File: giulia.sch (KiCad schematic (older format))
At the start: 128 parts, among them J1 AVR-ISP-6, SW1 RESET, SW2 BOOT, U1 ATmega32A-PU, Y1 16 MHz

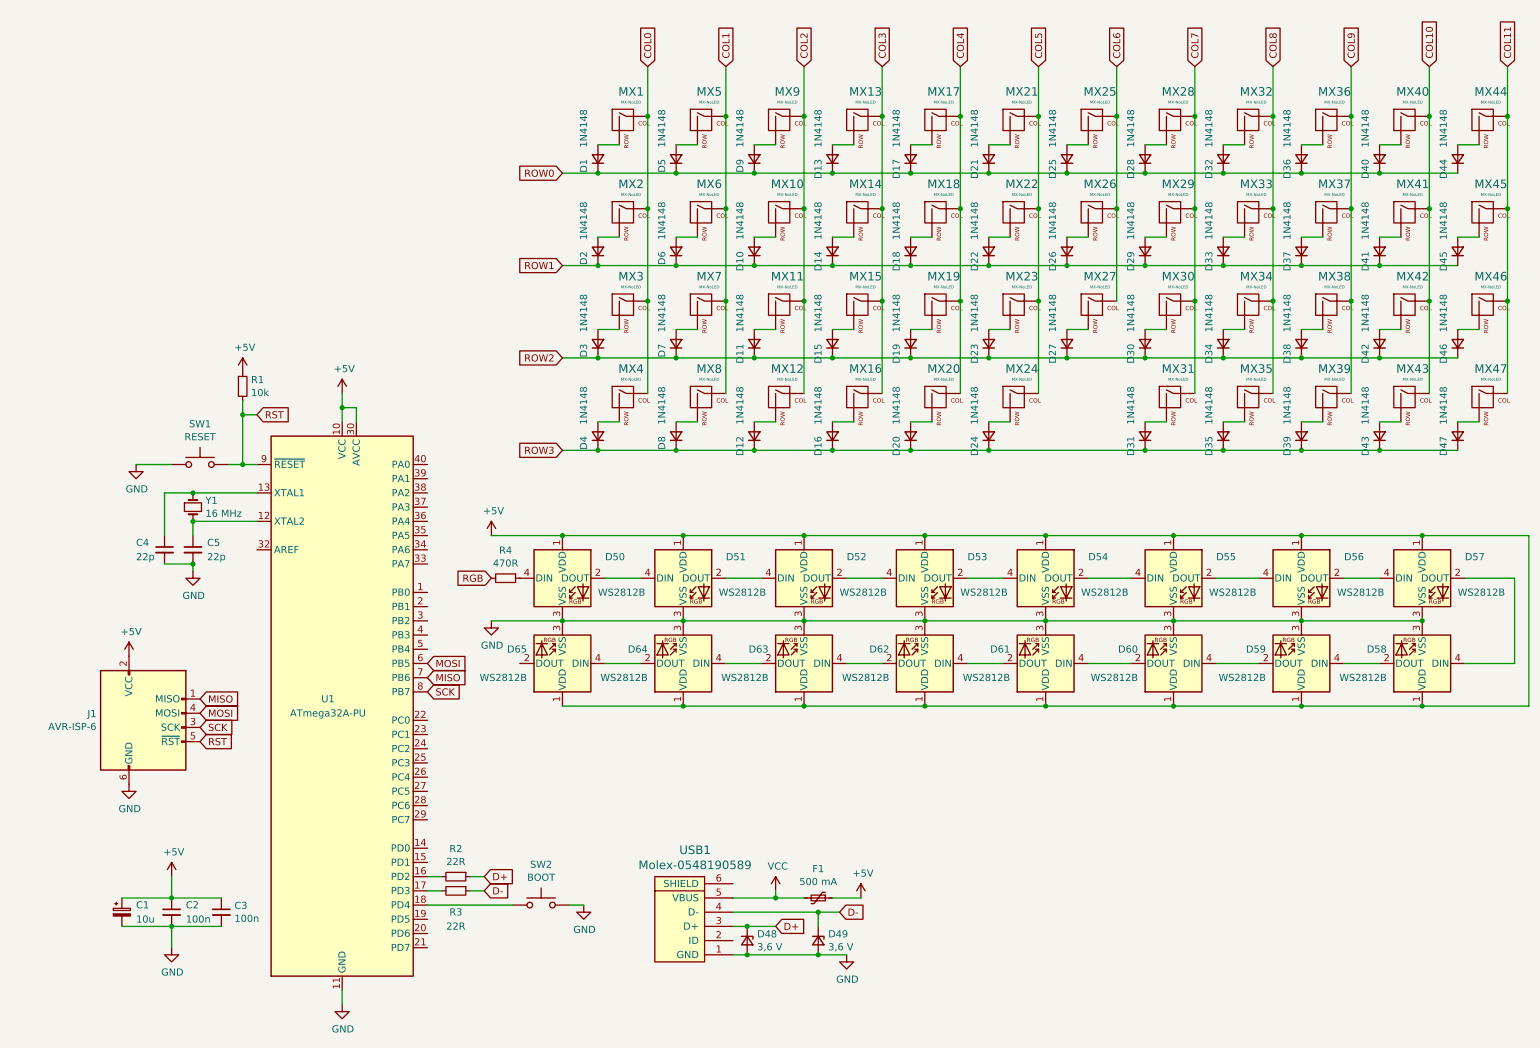
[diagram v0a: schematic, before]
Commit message: minor adjustments
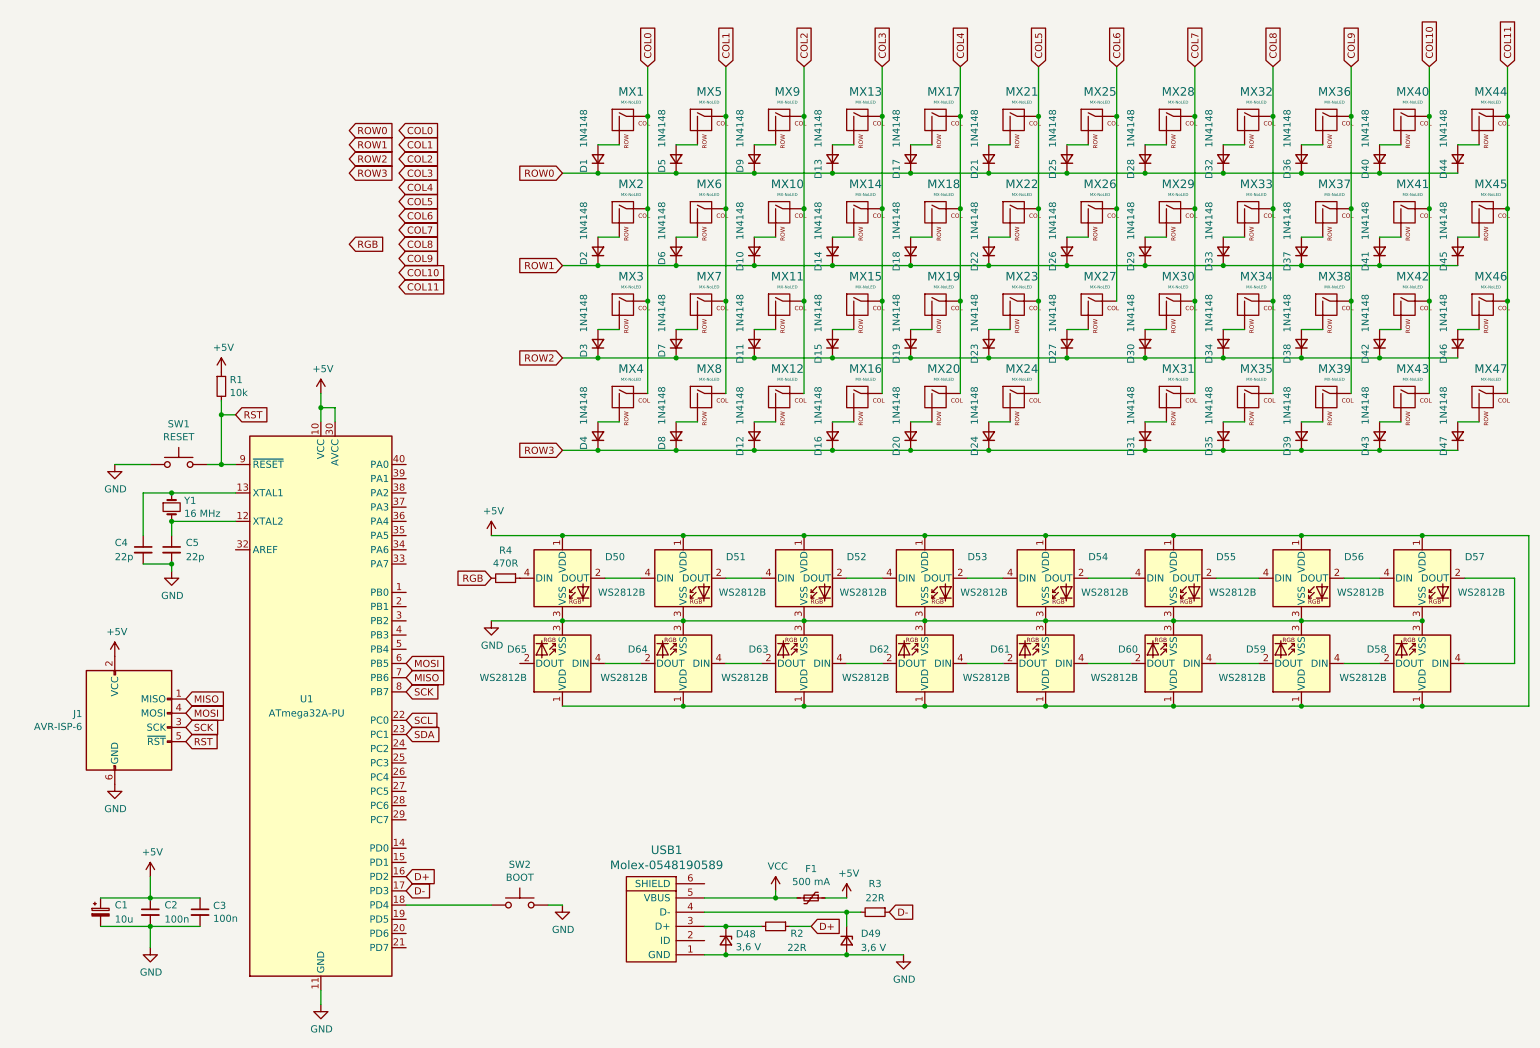
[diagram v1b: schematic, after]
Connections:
- net D+: now also U1.16 (PD2); no longer D48.1 (K), USB1.3 (D+)
- net D-: now also U1.17 (PD3); no longer D49.1 (K), USB1.4 (D-)
- net at R2.2: now also D48.1 (K), USB1.3 (D+); no longer U1.16 (PD2)
- net at R3.2: now also D49.1 (K), USB1.4 (D-); no longer U1.17 (PD3)
- net SCL: now reaches U1.22 (PC0)
- net SDA: now reaches U1.23 (PC1)
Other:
- moved on the sheet: C1, C2, C3, C4, C5, D48, D49, F1, J1, R1, R2, R3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

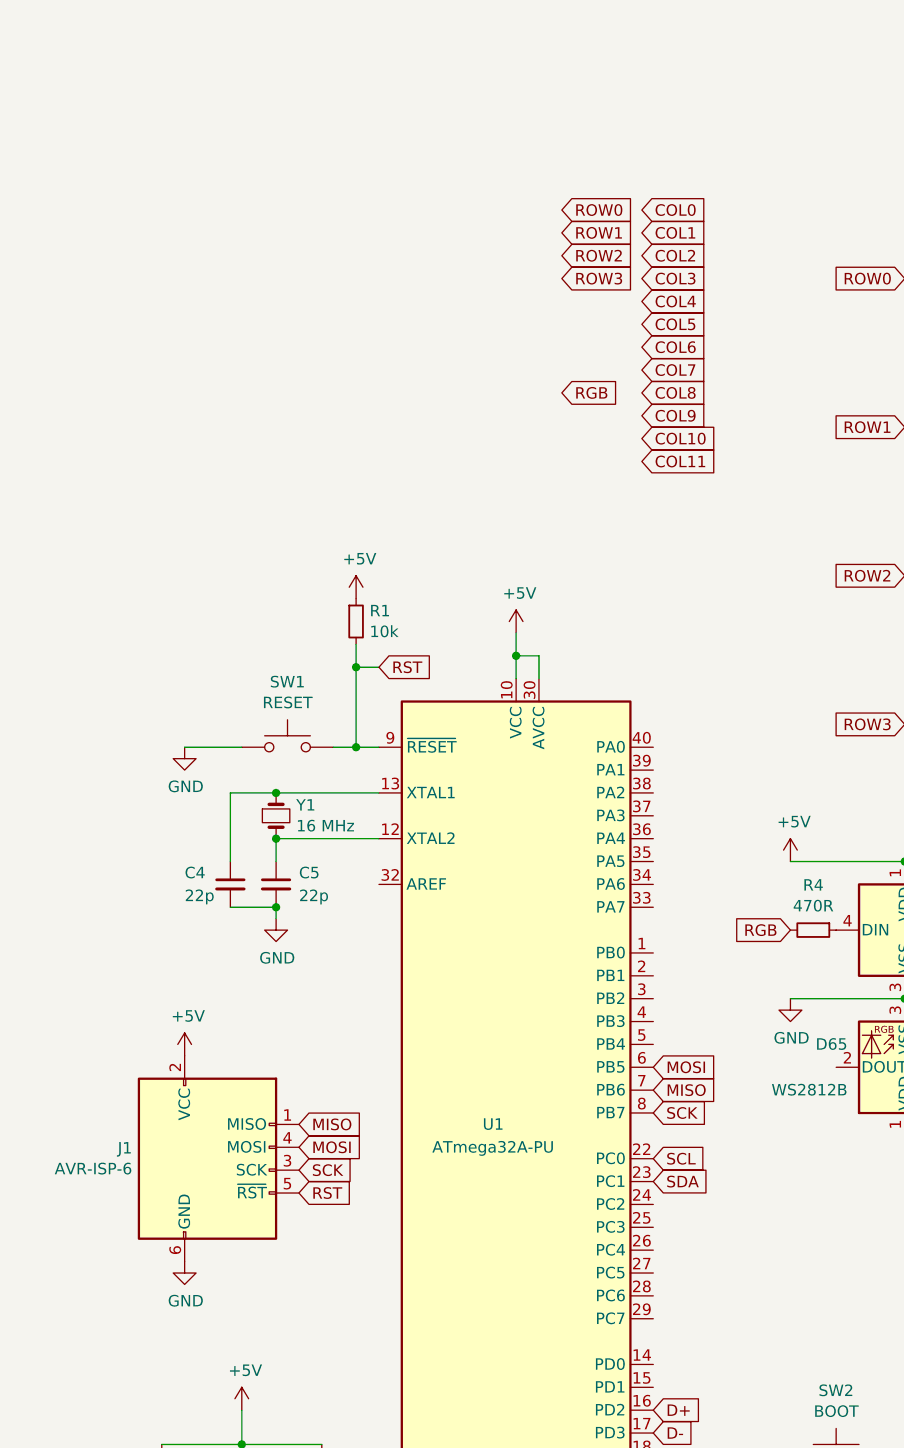
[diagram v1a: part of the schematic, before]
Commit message: schema hopefully complete
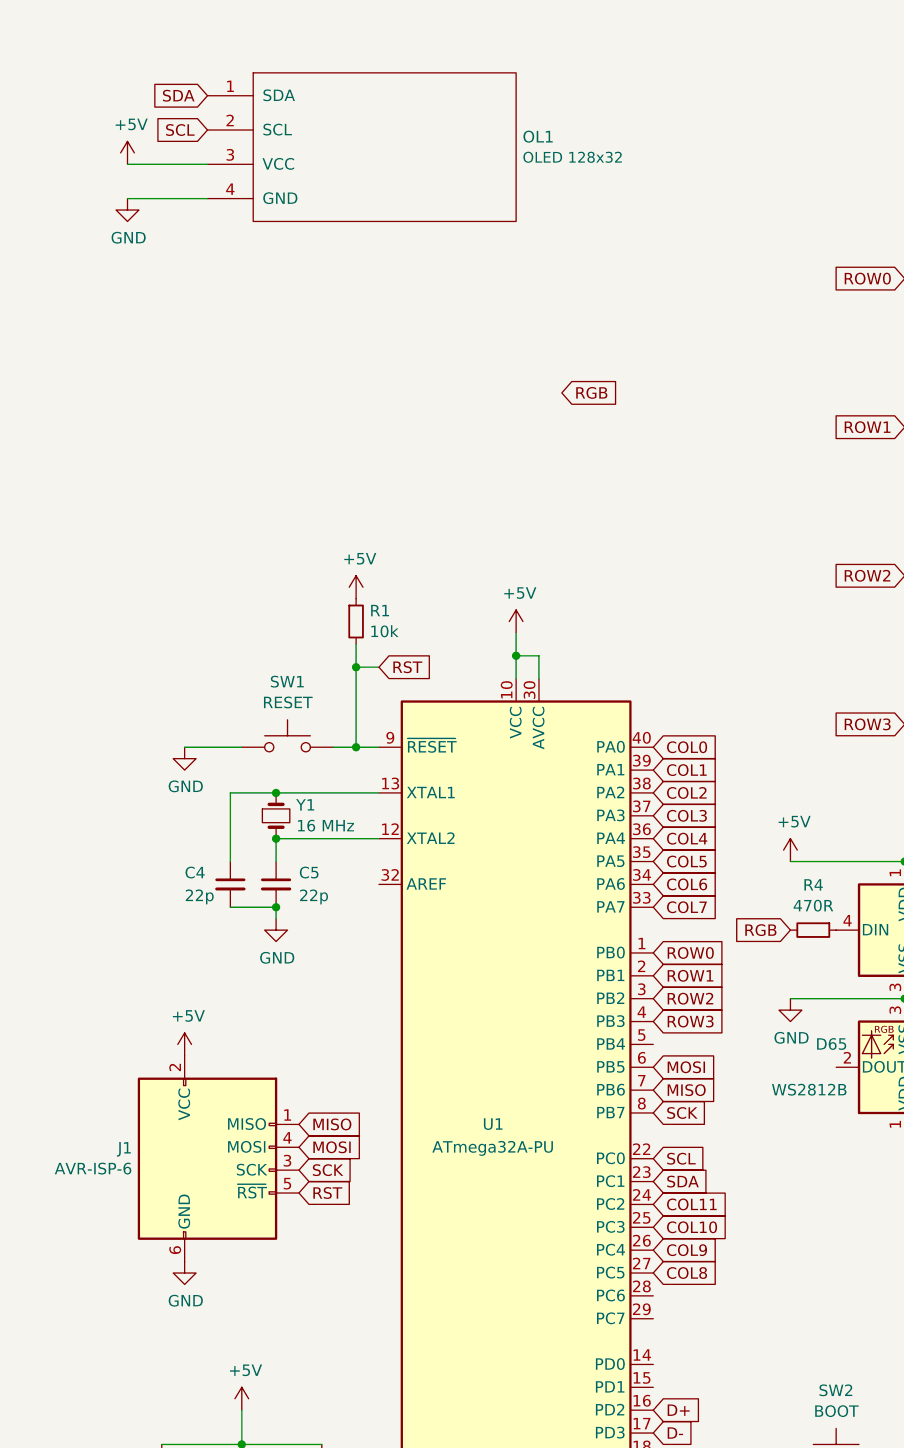
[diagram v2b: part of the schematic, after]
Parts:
- added OL1: OLED 128x32, symbol kbd:OLED
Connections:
- net +5V: now also OL1.3 (VCC)
- net COL0: now also U1.40 (PA0)
- net COL1: now also U1.39 (PA1)
- net COL10: now also U1.25 (PC3)
- net COL11: now also U1.24 (PC2)
- net COL2: now also U1.38 (PA2)
- net COL3: now also U1.37 (PA3)
- net COL4: now also U1.36 (PA4)
- net COL5: now also U1.35 (PA5)
- net COL6: now also U1.34 (PA6)
- net COL7: now also U1.33 (PA7)
- net COL8: now also U1.27 (PC5)
- net COL9: now also U1.26 (PC4)
- net GND: now also OL1.4 (GND)
- net ROW0: now also U1.1 (PB0)
- net ROW1: now also U1.2 (PB1)
- net ROW2: now also U1.3 (PB2)
- net ROW3: now also U1.4 (PB3)
- net SCL: now also OL1.2 (SCL)
- net SDA: now also OL1.1 (SDA)
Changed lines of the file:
@@
 Wire Wire Line
 	5950 6950 6100 6950
-Text GLabel 2850 1350 2    50   Input ~ 0
+Text GLabel 3250 4600 2    50   Input ~ 0
 ROW0
-Text GLabel 2850 1450 2    50   Input ~ 0
+Text GLabel 3250 4700 2    50   Input ~ 0
 ROW1
-Text GLabel 2850 1550 2    50   Input ~ 0
+Text GLabel 3250 4800 2    50   Input ~ 0
 ROW2
-Text GLabel 2850 1650 2    50   Input ~ 0
+Text GLabel 3250 4900 2    50   Input ~ 0
 ROW3
-Text GLabel 3200 1350 2    50   Input ~ 0
+Text GLabel 3250 3700 2    50   Input ~ 0
 COL0
-Text GLabel 3200 1450 2    50   Input ~ 0
+Text GLabel 3250 3800 2    50   Input ~ 0
 COL1
-Text GLabel 3200 1550 2    50   Input ~ 0
+Text GLabel 3250 3900 2    50   Input ~ 0
 COL2
-Text GLabel 3200 1650 2    50   Input ~ 0
+Text GLabel 3250 4000 2    50   Input ~ 0
 COL3
-Text GLabel 3200 1750 2    50   Input ~ 0
+Text GLabel 3250 4100 2    50   Input ~ 0
 COL4
-Text GLabel 3200 1850 2    50   Input ~ 0
+Text GLabel 3250 4200 2    50   Input ~ 0
 COL5
-Text GLabel 3200 1950 2    50   Input ~ 0
+Text GLabel 3250 4300 2    50   Input ~ 0
 COL6
-Text GLabel 3200 2050 2    50   Input ~ 0
+Text GLabel 3250 4400 2    50   Input ~ 0
 COL7
-Text GLabel 3200 2150 2    50   Input ~ 0
+Text GLabel 3250 6000 2    50   Input ~ 0
 COL8
-Text GLabel 3200 2250 2    50   Input ~ 0
+Text GLabel 3250 5900 2    50   Input ~ 0
 COL9
-Text GLabel 3200 2350 2    50   Input ~ 0
+Text GLabel 3250 5800 2    50   Input ~ 0
 COL10
-Text GLabel 3200 2450 2    50   Input ~ 0
+Text GLabel 3250 5700 2    50   Input ~ 0
 COL11
 Text GLabel 2850 2150 2    50   Input ~ 0
@@
 Text GLabel 3250 5600 2    50   Input ~ 0
 SDA
+$Comp
+L kbd:OLED OL1
+U 1 1 615D634B
+P 2050 1100
+F 0 "OL1" H 2678 1169 51  0000 L CNN
+F 1 "OLED 128x32" H 2678 1079 47  0000 L CNN
+F 2 "" H 2050 1200 60  0001 C CNN
+F 3 "" H 2050 1200 60  0001 C CNN
+	1    2050 1100
+	1    0    0    -1
+$EndComp
+Text GLabel 1300 1000 0    50   Input ~ 0
+SCL
+Text GLabel 1300 850  0    50   Input ~ 0
+SDA
+$Comp
+L power:+5V #PWR?
+U 1 1 615D9D0C
+P 950 1150
+F 0 "#PWR?" H 950 1000 50  0001 C CNN
+F 1 "+5V" H 965 1323 50  0000 C CNN
+F 2 "" H 950 1150 50  0001 C CNN
+F 3 "" H 950 1150 50  0001 C CNN
+	1    950  1150
+	1    0    0    -1
+$EndComp
+Wire Wire Line
+	950  1150 1300 1150
+$Comp
+L power:GND #PWR?
+U 1 1 615EB060
+P 950 1300
+F 0 "#PWR?" H 950 1050 50  0001 C CNN
+F 1 "GND" H 955 1127 50  0000 C CNN
+F 2 "" H 950 1300 50  0001 C CNN
+F 3 "" H 950 1300 50  0001 C CNN
+	1    950  1300
+	1    0    0    -1
+$EndComp
+Wire Wire Line
+	950  1300 1300 1300
 $EndSCHEMATC
